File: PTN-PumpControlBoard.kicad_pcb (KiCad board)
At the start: 2 copper layers, 100.2 x 72 mm, 43 parts, among them J1 PeripheralCANConnector, Q1 NMOS, Q2 NMOS, Q3 NMOS, SW1 SW_Push, SW2 SW_Push, SW3 SW_Push, U1 EMC2305-1-AP-TR, U2 PeripheralSOM, U3 ST7735R

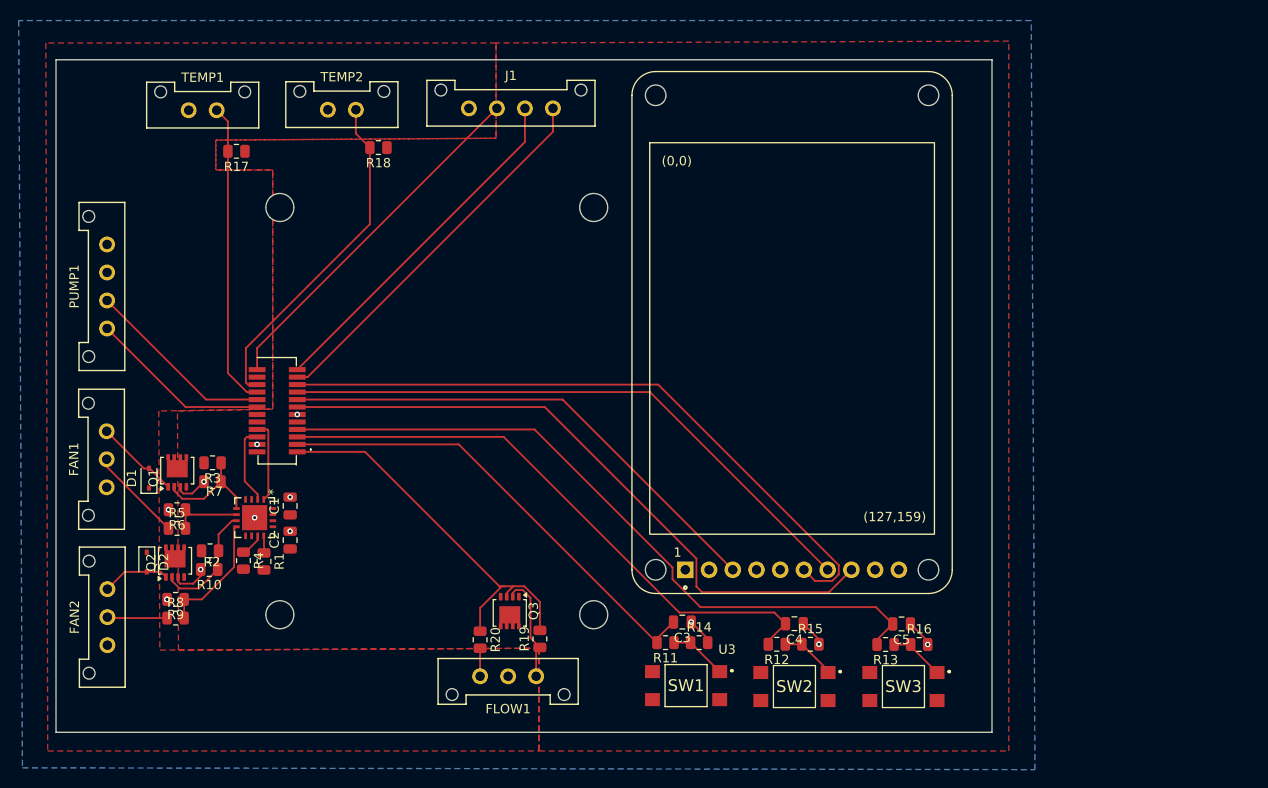
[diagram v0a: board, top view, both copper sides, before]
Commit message: Initial layout with 1 pump, 2 temp, 1 flow all on front side
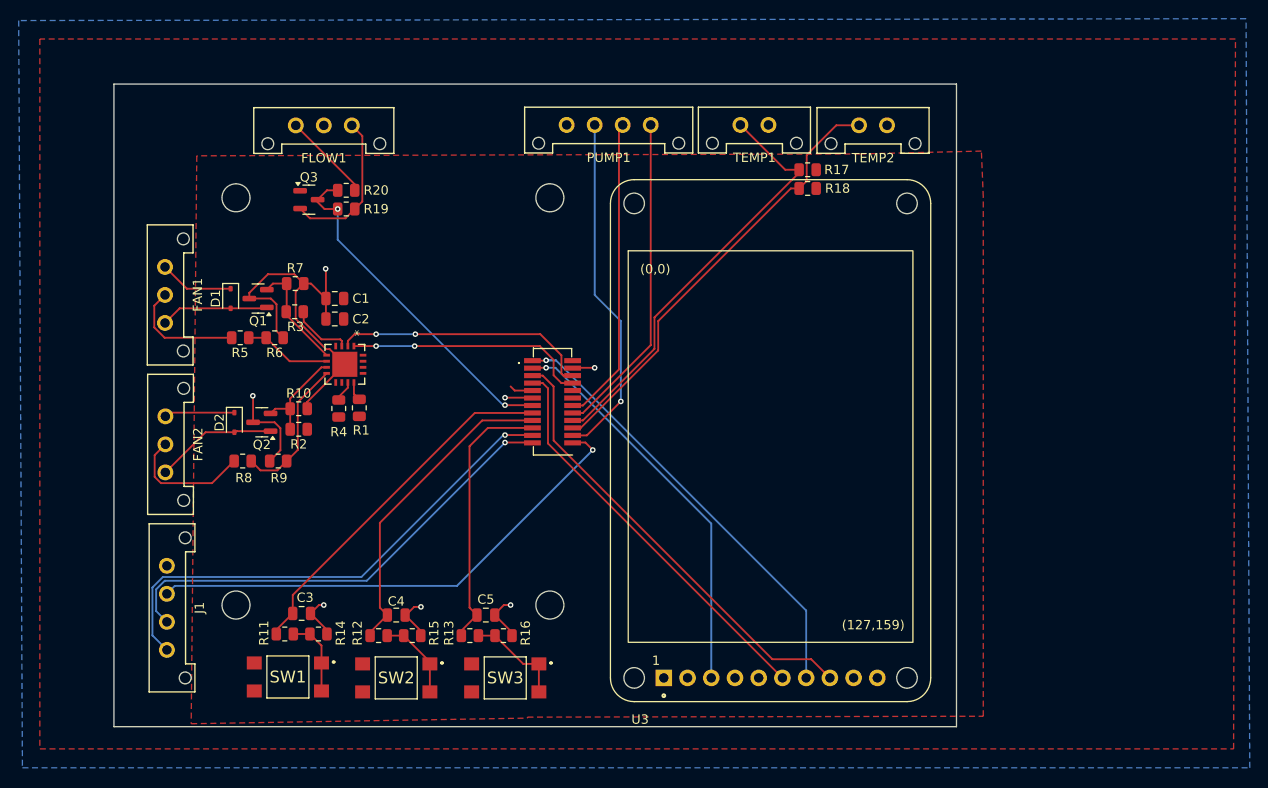
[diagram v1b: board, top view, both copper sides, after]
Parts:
- Q1, Q2, Q3: footprint Package_TO_SOT_SMD:LFPAK33 -> Package_TO_SOT_SMD:SOT-23
- moved FLOW1 62.2 mm to (135.4, 71.2)
- moved PUMP1 62.2 mm to (167.4, 71.2), turned to 180 degrees
- moved TEMP1 62.1 mm to (180.0, 71.2), turned to 180 degrees
- moved R17 61.2 mm to (184.2, 76.0)
- moved TEMP2 59.9 mm to (192.7, 71.2), turned to 180 degrees
- moved J1 58.7 mm to (115.6, 118.4), turned to -90 degrees
- moved R19 50.5 mm to (134.8, 80.2), turned to 180 degrees
- moved R20 50.2 mm to (134.8, 78.2), turned to 0 degrees
- moved Q3 49.0 mm to (130.8, 79.2), turned to 0 degrees
- moved R18 46.2 mm to (184.2, 78.0)
- moved C5 44.5 mm to (149.7, 123.7)
- moved R13 44.5 mm to (148.0, 125.9)
- moved R16 44.5 mm to (151.6, 125.9)
- moved C4 42.6 mm to (140.2, 123.7)
- moved R15 42.6 mm to (141.9, 125.9)
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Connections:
- R18 pad 1: +3V3 -> +3.3V
- U2 pad 1: /FLOW -> /MOSI
- U2 pad 13: /SCLK -> /FLOW
- U2 pad 14: /PUMP_PG -> /PUMP_PWM
- U2 pad 15: /LCD_RESET -> /FAN_SPEED
- U2 pad 16: /PUMP_PWM -> /PUMP_PG
- U2 pad 17: /MOSI -> /PUMP_SPEED
- U2 pad 19: /LCD_TFT_~{CS} -> /SYST_MODE
- U2 pad 3: /FAN_SPEED -> /LCD_RESET
- U2 pad 5: /PUMP_SPEED -> /SCLK
- U2 pad 7: /SYST_MODE -> /LCD_TFT_~{CS}
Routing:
- net GND: track 19.4 -> 80.4 mm, vias 13 -> 7
- net +12V: track 0.00 -> 53.0 mm, vias 0 -> 1
- net /SYST_MODE: track 76.0 -> 28.9 mm
- net /PUMP_SPEED: track 63.2 -> 34.1 mm
- net /LCD_TFT_~{CS}: track 71.5 -> 43.3 mm
- net /SCLK: track 70.3 -> 48.6 mm
- net /FAN_SDA: track 8.46 -> 27.9 mm, vias 0 -> 2
- net /FAN_SCL: track 8.84 -> 26.4 mm, vias 0 -> 2
- net /MOSI: track 64.7 -> 48.6 mm, vias 0 -> 1
- net GNDPWR: track 38.6 -> 54.6 mm, vias 0 -> 1
- net /PUMP_PG: track 19.5 -> 34.9 mm
- net CAN_L: track 40.8 -> 54.9 mm, vias 0 -> 1
- net /TEMP1: track 32.6 -> 45.8 mm
- net CAN_H: track 38.1 -> 50.9 mm, vias 0 -> 1
- net /PUMP_PWM: track 20.5 -> 32.9 mm
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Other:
- board size 100.2 x 72 mm -> 90.2 x 68.8 mm
